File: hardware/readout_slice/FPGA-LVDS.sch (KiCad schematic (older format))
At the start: 12 parts

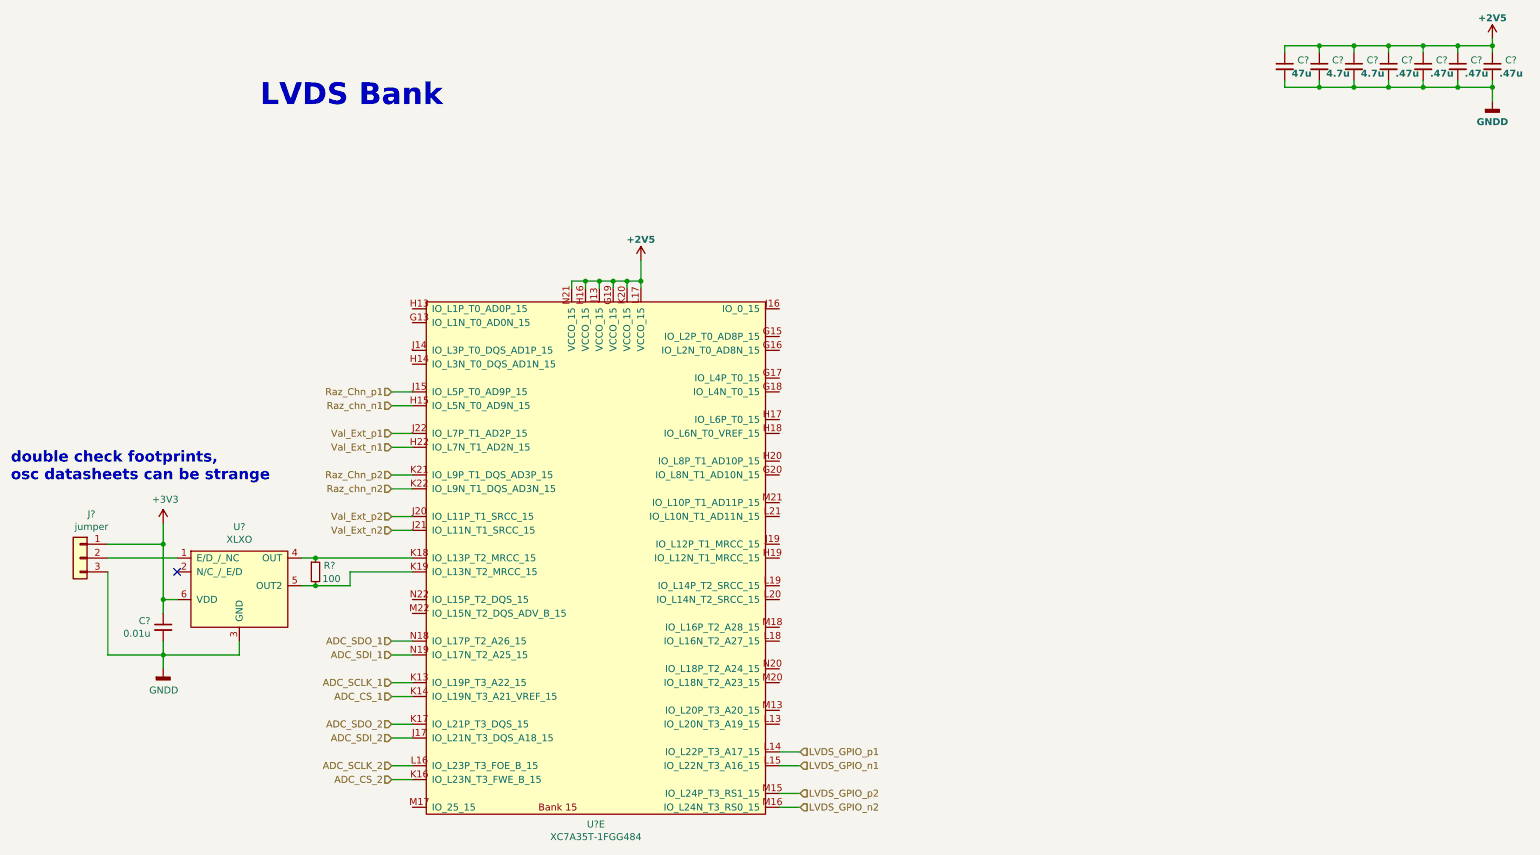
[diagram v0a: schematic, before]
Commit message: auto push run at Wed Apr 28 10:36:58 EDT 2021
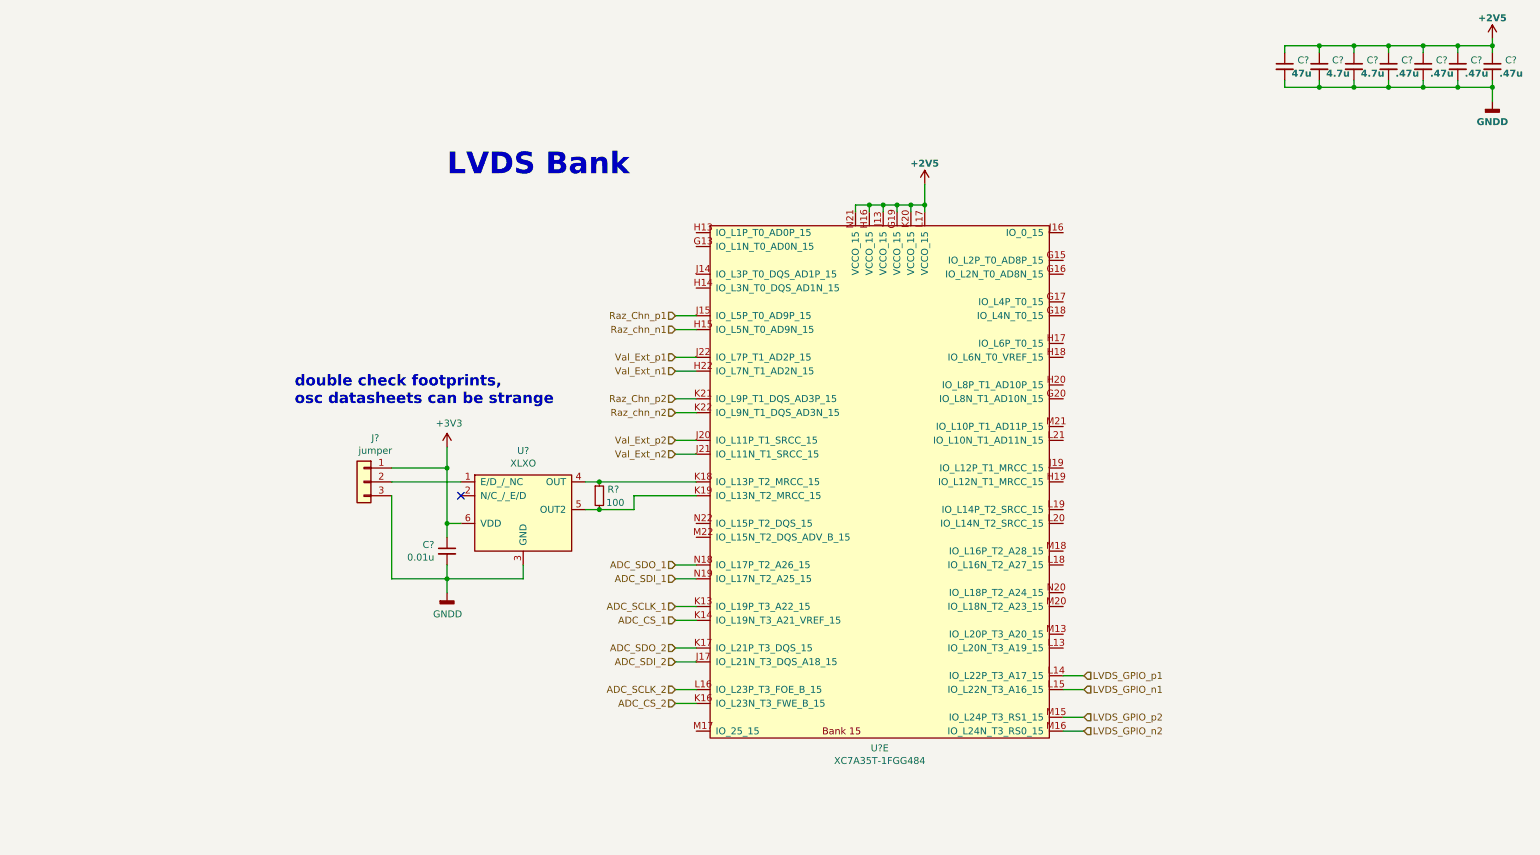
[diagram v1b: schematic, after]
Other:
- moved on the sheet: C?, J?, R?, U?, U?E
